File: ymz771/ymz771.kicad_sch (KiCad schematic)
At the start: 94 parts, among them IC1 CH221K, J1 Conn_01x04_Pin, J2 Conn_02x12_Counter_Clockwise, J3 Conn_01x08_Pin, J4 Conn_02x08_Counter_Clockwise, J5 Conn_01x04_Pin, J6 Conn_01x05_Pin, J7 USB_C_Receptacle_PowerOnly_6P, J8 Conn_01x10_Pin, SW1 SW_DIP_x04, Y1 Crystal

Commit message: commit2605161301
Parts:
- removed C10, C7, C8, C9: C_Polarized_Small, Capacitor_THT:CP_Radial_D6.3mm_P2.50mm, symbol Device:C_Polarized_Small
- removed C15, C16: C_Polarized_Small, Capacitor_THT:CP_Radial_D8.0mm_P3.50mm, symbol Device:C_Polarized_Small
- removed D1, D2, D3, D4, D5: LED_Small, LED_SMD:LED_0603_1608Metric_Pad1.05x0.95mm_HandSolder, symbol Device:LED_Small
- removed IC1: CH221K, YMZ771:SOT95P280X120-6N, symbol Yamaha:CH221K
- removed J1: Conn_01x04_Pin, Connector_PinHeader_2.54mm:PinHeader_1x04_P2.54mm_Vertical, symbol Connector:Conn_01x04_Pin
- removed J3: Conn_01x08_Pin, Connector_PinHeader_2.54mm:PinHeader_1x08_P2.54mm_Vertical, symbol Connector:Conn_01x08_Pin
- removed J5: Conn_01x04_Pin, Connector_PinSocket_2.54mm:PinSocket_1x04_P2.54mm_Vertical, symbol Connector:Conn_01x04_Pin
- removed J6: Conn_01x05_Pin, Connector_PinHeader_2.54mm:PinHeader_1x05_P2.54mm_Vertical, symbol Connector:Conn_01x05_Pin
- removed J7: USB_C_Receptacle_PowerOnly_6P, Connector_USB:USB_C_Receptacle_GCT_USB4125-xx-x_6P_TopMnt_Horizontal, symbol Connector:USB_C_Receptacle_PowerOnly_6P
- removed J8: Conn_01x10_Pin, Connector_PinHeader_2.54mm:PinHeader_1x10_P2.54mm_Vertical, symbol Connector:Conn_01x10_Pin
- removed R1, R12, R17, R2, R21, R22, R23, R24, R25, R26, R27, R28, R29, R3, R30, R31, R32, R37, R4, R9: 10k, Resistor_SMD:R_0603_1608Metric_Pad0.98x0.95mm_HandSolder, symbol Device:R_Small
- removed R33: 1k, Resistor_SMD:R_0603_1608Metric_Pad0.98x0.95mm_HandSolder, symbol Device:R_Small
- removed R34, R35: 5.1k, Resistor_SMD:R_0603_1608Metric_Pad0.98x0.95mm_HandSolder, symbol Device:R_Small
- removed R36, R38, R39, R40, R41, R44, R45, R46, R47, R48, R49, R50: 100k, Resistor_SMD:R_0603_1608Metric_Pad0.98x0.95mm_HandSolder, symbol Device:R_Small
- removed SW1: SW_DIP_x04, Button_Switch_SMD:SW_DIP_SPSTx04_Slide_KingTek_DSHP04TS_W7.62mm_P1.27mm, symbol Switch:SW_DIP_x04
- removed U1: ~, YMZ771:YMZ771-F, symbol Yamaha:YMZ771
- removed Y1: Crystal, Crystal:Crystal_SMD_HC49-SD, symbol Device:Crystal
- added C10, C11, C12, C2, C3: 0.1uF, Capacitor_SMD:C_0603_1608Metric, symbol Device:C_Small
- added C14, C15: 2.2nF, Capacitor_SMD:C_0603_1608Metric, symbol Device:C_Small
- added C16, C20: 2.2uF, Capacitor_SMD:C_0603_1608Metric, symbol Device:C_Small
- added C17: 4u7, Capacitor_SMD:C_0603_1608Metric, symbol Device:C
- added C18, C21, C5, C6: 0.1u, Capacitor_SMD:C_0603_1608Metric, symbol Device:C_Small
- added C19, C22, C8, C9: 47u, Capacitor_SMD:C_0603_1608Metric, symbol Device:C_Small
- added C31, C32: C_Small, Capacitor_SMD:C_0603_1608Metric, symbol Device:C_Small
- added C33, C34: 10uF, Capacitor_SMD:C_1812_4532Metric, symbol Device:C_Small
- added C7: 0u1, Capacitor_SMD:C_0603_1608Metric, symbol Device:C
- added D1: LED, LED_SMD:LED_0603_1608Metric, symbol Device:LED
- added D12, D13, D14, D15, D16, D17, D18, D19: LED_Small, LED_SMD:LED_0603_1608Metric_Pad1.05x0.95mm_HandSolder, symbol Device:LED_Small
- added J1: YMZ771-F, QFP80P1880X2480X295-80N, symbol Yamaha:YMZ771-F
- added J2: Micro_SD_Card_Det2, Connector_Card:microSD_HC_Hirose_DM3AT-SF-PEJM5, symbol Connector:Micro_SD_Card_Det2
- added J4: MJ-8435, YMZ771:MJ-8435, symbol Yamaha:MJ-8435
- added J7: USB_C_Receptacle_USB2.0_16P, Connector_USB:USB_C_Receptacle_GCT_USB4105-xx-A_16P_TopMnt_Horizontal, symbol Connector:USB_C_Receptacle_USB2.0_16P
- added J8: Conn_01x02_Pin, Connector_PinHeader_2.54mm:PinHeader_1x02_P2.54mm_Vertical, symbol Connector:Conn_01x02_Pin
- added J9: Conn_02x06_Counter_Clockwise, Connector_PinHeader_1.27mm:PinHeader_2x06_P1.27mm_Vertical_SMD, symbol Connector_Generic:Conn_02x06_Counter_Clockwise
- added Q1, Q2, Q3, Q4: NMOS, Package_TO_SOT_SMD:SOT-23, symbol Transistor_FET_Other:Q_NMOS_Depletion_GSD
- added R1, R3, R4: 5k1, Resistor_SMD:R_0603_1608Metric, symbol Device:R
- added R12, R9: 470, Resistor_SMD:R_0603_1608Metric, symbol Device:R
- added R17: 10k, Resistor_SMD:R_0603_1608Metric, symbol Device:R
- added R55, R56: 10k, Resistor_SMD:R_0603_1608Metric, symbol Device:R_Small
- added RN1, RN10, RN11, RN12, RN13, RN14, RN2, RN3, RN4, RN5, RN6, RN7, RN8, RN9: R_Pack04, Yamaha:MNR04M0ABJ, symbol Device:R_Pack04
- added SW1: SW_Push, footprints:SKRPABE010, symbol Switch:SW_Push
- added SW2: RotaryEncoder, Rotary_Encoder:RotaryEncoder_Bourns_Horizontal_PEC09-2xxxF-Nxxxx, symbol Device:RotaryEncoder
- added SW3: SW_MEC_5E, Yamaha:SW_SKRPABE010, symbol Switch:SW_MEC_5E
- added U1: TS5A23159DGS, Package_SO:VSSOP-10_3x3mm_P0.5mm, symbol Analog_Switch:TS5A23159DGS
- added U10: ESP32-S3-WROOM-1, RF_Module:ESP32-S3-WROOM-1, symbol RF_Module:ESP32-S3-WROOM-1
- added U11, U12: 74AHC541, Package_SO:SSOP-20_5.3x7.2mm_P0.65mm, symbol 74xx:74AHC541
- added U13, U14: (no value), Package_DIP:DIP-8_W7.62mm, symbol Yamaha:PAM8012
- added U2, U5: TXS0104EPW, Package_SO:TSSOP-14_4.4x5mm_P0.65mm, symbol Logic_LevelTranslator:TXS0104EPW
- added U3: (no value), Package_TO_SOT_SMD:TSOT-23-5_HandSoldering, symbol Yamaha:rt9080
- added U4: CH340K, Package_SO:SSOP-10-1EP_3.9x4.9mm_P1mm_EP2.1x3.3mm, symbol Interface_USB:CH340K
- added U6: (no value), YMZ771:OSL2051A-LR, symbol Yamaha:OSL2051A
- added U7: 74HC595, Package_SO:TSSOP-16_4.4x5mm_P0.65mm, symbol 74xx:74HC595
- added U8: PCM5102A, Package_SO:TSSOP-20_4.4x6.5mm_P0.65mm, symbol Audio:PCM5102A
- added Y1: 16.384MHz, Crystal:Crystal_SMD_3225-4Pin_3.2x2.5mm, symbol Device:Crystal_GND24
- C13: value C_Small -> 0.1uF
- J10: renamed from J4; footprint Connector_PinHeader_2.54mm:PinHeader_2x08_P2.54mm_Vertical -> Connector_PinHeader_1.27mm:PinHeader_2x08_P1.27mm_Vertical_SMD
- J11: renamed from J2; footprint Connector_PinHeader_2.54mm:PinHeader_2x12_P2.54mm_Vertical -> Connector_PinHeader_1.27mm:PinHeader_2x12_P1.27mm_Vertical_SMD
- R10, R13, R14, R15, R16, R6, R7, R8: value 10k -> R_Small; footprint Resistor_SMD:R_0603_1608Metric_Pad0.98x0.95mm_HandSolder -> Resistor_SMD:R_0603_1608Metric
- R11, R18, R19, R20, R5: footprint Resistor_SMD:R_0603_1608Metric_Pad0.98x0.95mm_HandSolder -> Resistor_SMD:R_0603_1608Metric
- R51: value 100k -> 1M; footprint Resistor_SMD:R_0603_1608Metric_Pad0.98x0.95mm_HandSolder -> Resistor_SMD:R_0603_1608Metric
- renumbered C6 to C23, C1 to C24, C2 to C25, C14 to C26, C5 to C27, C11 to C28, C12 to C29, C3 to C30, C4 to C35, D7 to D2, D6 to D3, D12 to D4, D13 to D5, D14 to D6, D15 to D7, R43 to R37, R42 to R57
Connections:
- net AVDD is gone; now on net +5V: C25.1
- net VDD1 is gone; now on net +5V: C24.1, R57.2
- net VDD2 is gone; now on net +5V: C27.1, C35.1
- net VDD4 is gone; now on net +5V: C23.1, C28.1
- net /CS is gone; now on an unnamed net: R51.2
- net +5V: now also D2.2 (A), R11.2, R19.2, C10.1, C17.1, C3.2, C33.1, C34.1, C5.2, J1.16 (VDD1), J1.25 (AVDD), J1.28 (~{TEST0}), J1.29 (~{TEST1}), J1.30 (VDD5), J1.37 (~{TEST2}), J1.38 (VDD2), J1.55 (VDD3), J1.72 (VDD4), J7.A4 (VBUS), J7.A9 (VBUS), J7.B4 (VBUS), J7.B9 (VBUS), J8.1 (Pin_1), R1.1, R55.2, R56.2, RN12.5 (R4.2), RN12.6 (R3.2), RN12.7 (R2.2), RN12.8 (R1.2), RN7.5 (R4.2), RN7.6 (R3.2), RN7.7 (R2.2), RN7.8 (R1.2), U1.8 (VCC), U11.20 (VCC), U12.20 (VCC), U13.1 (Vin), U14.1 (Vin), U2.14 (V_{CCB}), U3.1 (Vin), U3.3 (EN), U4.7 (VCC), U5.14 (V_{CCB}), U7.16 (VCC)
- net AD: now also J1.12 (AD), RN8.1 (R1.1), U12.2 (A0)
- net AOL: now also J1.23 (AOL), U1.9
- net AOR: now also J1.24 (AOR), U1.7
- net BCO: now also J1.31 (BCO), U5.11 (B3)
- net CLKO: now also J1.34 (CLKO), U5.10 (B4)
- net ENA: now also J1.13 (ENA), RN8.2 (R2.1), U12.3 (A1)
- net GND: now also R18.1, C10.2, C11.1, C12.2, C14.1, C15.1, C17.2, C18.1, C19.1, C2.1, C20.1, C21.2, C22.2, C3.1, C31.2, C32.2, C33.2, C34.2, C5.1, C6.1, C7.1, C8.1, C9.1, J1.17 (VSS1), J1.26 (AVSS), J1.39 (VSS2), J1.56 (VSS3), J1.73 (VSS4), J2.11 (SHIELD), J2.6 (VSS), J4.2 (2_1), J4.3 (2_2), J7.A1 (GND), J7.A12 (GND), J7.B1 (GND), J7.B12 (GND), J7.S1 (SHIELD), J8.2 (Pin_2), Q1.2 (S), Q2.2 (S), Q3.2 (S), R17.2, R3.1, R4.2, RN1.5 (R4.2), RN1.6 (R3.2), RN1.7 (R2.2), RN1.8 (R1.2), RN10.5 (R4.2), RN10.6 (R3.2), RN10.7 (R2.2), RN10.8 (R1.2), RN11.5 (R4.2), RN11.6 (R3.2), RN11.7 (R2.2), RN11.8 (R1.2), RN13.5 (R4.2), RN13.6 (R3.2), RN13.7 (R2.2), RN13.8 (R1.2), RN14.5 (R4.2), RN14.6 (R3.2), RN14.7 (R2.2), RN14.8 (R1.2), RN2.5 (R4.2), RN2.6 (R3.2), RN2.7 (R2.2), RN2.8 (R1.2), RN3.5 (R4.2), RN3.6 (R3.2), RN3.7 (R2.2), RN3.8 (R1.2), RN4.5 (R4.2), RN4.6 (R3.2), RN4.7 (R2.2), RN4.8 (R1.2), RN5.5 (R4.2), RN5.6 (R3.2), RN5.7 (R2.2), RN5.8 (R1.2), RN6.5 (R4.2), RN6.6 (R3.2), RN6.7 (R2.2), RN6.8 (R1.2), RN8.5 (R4.2), RN8.6 (R3.2), RN8.7 (R2.2), RN8.8 (R1.2), RN9.5 (R4.2), RN9.6 (R3.2), RN9.7 (R2.2), RN9.8 (R1.2), SW1.1, SW2.C, SW3.3 (K), SW3.4 (A), U1.3 (GND), U10.1 (GND), U10.40 (GND), U10.41 (GND), U11.1 (G1), U11.10 (GND), U11.19 (G2), U12.1 (G1), U12.10 (GND), U12.19 (G2), U13.2 (GND), U13.4 (IN-), U13.5 (SPK-), U13.6 (SPK-), U14.2 (GND), U14.4 (IN-), U14.5 (SPK-), U14.6 (SPK-), U2.7 (GND), U3.2 (GND), U4.11 (GND), U4.3 (GND), U5.7 (GND), U7.8 (GND), U8.10 (DEMP), U8.11 (FLT), U8.16 (FMT), U8.19 (DGND), U8.3 (CPGND), U8.9 (AGND), Y1.2, Y1.4; no longer D10.1 (K), D11.1 (K), D2.1 (K), D4.1 (K), D5.1 (K), D6.1 (K), D7.1 (K), D8.1 (K), D9.1 (K), R10.2, R11.2, R13.2, R14.2, R15.2, R16.2, R18.2, R19.2, R20.2, R5.2, R6.2, R7.2, R8.2
- net LRO: now also J1.32 (LRO), U5.13 (B1)
- net MA00: now also J1.65 (MA00), RN1.1 (R1.1)
- net MA01: now also J1.64 (MA01), RN1.2 (R2.1)
- net MA02: now also J1.63 (MA02), RN1.3 (R3.1)
- net MA03: now also J1.62 (MA03), RN1.4 (R4.1)
- net MA04: now also J1.61 (MA04), RN2.1 (R1.1); no longer R5.1
- net MA05: now also J1.60 (MA05), RN2.2 (R2.1); no longer R6.1
- net MA06: now also J1.59 (MA06), RN2.3 (R3.1); no longer R7.1
- net MA07: now also J1.58 (MA07), RN2.4 (R4.1); no longer R8.1
- net MA08: now also J1.57 (MA08), RN3.1 (R1.1)
- net MA09: now also J1.54 (MA09), RN3.2 (R2.1); no longer R10.1
- net MA10: now also J1.53 (MA10), RN3.3 (R3.1); no longer R11.1
- net MA11: now also J1.52 (MA11), RN3.4 (R4.1)
- net MA12: now also J1.51 (MA12), RN4.1 (R1.1); no longer R13.1
- net MA13: now also J1.50 (MA13), RN4.2 (R2.1); no longer R14.1
- net MA14: now also J1.49 (MA14), RN4.3 (R3.1); no longer R15.1
- net MA15: now also J1.48 (MA15), RN4.4 (R4.1); no longer R16.1
- net MA16: now also J1.47 (MA16), RN5.1 (R1.1)
- net MA17: now also J1.46 (MA17), RN5.2 (R2.1); no longer R18.1
- net MA18: now also J1.45 (MA18), RN5.3 (R3.1); no longer R19.1
- net MA19: now also J1.44 (MA19), RN5.4 (R4.1); no longer R20.1
- net MA20: now also J1.43 (MA20), RN6.1 (R1.1)
- net MA21: now also J1.42 (MA21), RN6.2 (R2.1)
- net MA22: now also J1.41 (MA22), RN6.3 (R3.1)
- net MA23: now also J1.40 (MA23), RN6.4 (R4.1)
- net MBMD: now also J1.20 (MBMD), RN7.3 (R3.1), U12.8 (A6)
- net MD00: now also J1.3 (MD00)
- net MD01: now also J1.2 (MD01)
- net MD02: now also J1.1 (MD02)
- net MD03: now also J1.80 (MD03)
- net MD04: now also J1.79 (MD04)
- net MD05: now also J1.78 (MD05)
- net MD06: now also J1.77 (MD06)
- net MD07: now also J1.76 (MD07)
- net MD08: now also J1.75 (MD08)
- net MD09: now also J1.74 (MD09)
- net MD10: now also J1.71 (MD10)
- net MD11: now also J1.70 (MD11)
- net MD12: now also J1.69 (MD12)
- net MD13: now also J1.68 (MD13)
- net MD14: now also J1.67 (MD14)
- net MD15: now also J1.66 (MD15)
- net SDO: now also J1.33 (SDO), U5.12 (B2)
- net +3V3: now reaches C13.1
- net +3V3: now also R20.2, C11.2, C12.1, C2.2, C21.1, C22.1, C6.2, C8.2, C9.2, J2.4 (VDD), Q4.1 (G), U10.2 (3V3), U2.1 (V_{CCA}), U2.8 (OE), U3.5 (Vout), U5.1 (V_{CCA}), U5.8 (OE), U8.1 (CPVDD), U8.20 (DVDD), U8.8 (AVDD)
- net at D9.2 (A): now also RN12.2 (R2.1)
- net at D6.2 (A): now also U12.16 (Y2)
- net at D10.2 (A): now also RN12.3 (R3.1)
- net at C30.1: now also R51.1, J1.36 (XI), Y1.1
- net at D4.2 (A): now also U12.18 (Y0)
- net at C29.1: now also J1.35 (XO), Y1.3
- net at R37.1: now also D2.1 (K); no longer D2.2 (A)
- net at D8.2 (A): now also RN12.1 (R1.1)
- net at D11.2 (A): now also RN12.4 (R4.1)
- net at D5.2 (A): now also U12.17 (Y1)
- net at D7.2 (A): now also U12.15 (Y3); no longer R51.1
- net Vref: no longer names the net of C26.1
- net Vref: now also J1.27 (VREF)
- net /PLAY renamed /PLAY#
- net /PLAY#: now also R19.1, J1.22 (~{PLAY}), Q4.3 (D)
- new net: D19.1 (K), RN10.4 (R4.1)
- new net: D19.2 (A), U11.11 (Y7)
- new net: R9.2, U8.6 (OUTL)
- new net: R7.1, U7.1 (QB)
- new net: R7.2, U6.9 (B)
- new net: C20.2, U8.5 (VNEG)
- new net: R14.1, U7.5 (QF)
- new net: R14.2, U6.7 (F)
- new net: R6.1, U7.15 (QA)
- new net: R8.1, U7.2 (QC)
- new net: R10.1, U7.3 (QD)
- new net: R13.1, U7.4 (QE)
- new net: R15.1, U7.6 (QG)
- new net: R16.1, U7.7 (QH)
- new net: Q1.1 (G), R5.1
- new net: R10.2, U6.1 (D)
- new net: D6.1 (K), RN11.3 (R3.1)
- new net: D16.1 (K), RN10.1 (R1.1)
- new net: D16.2 (A), U11.14 (Y4)
- new net: J7.A5 (CC1), R3.2
- new net: J4.4 (3), U14.7 (SPK+), U14.8 (SPK+)
- new net: D12.1 (K), RN9.1 (R1.1)
- new net: D12.2 (A), U11.18 (Y0)
- new net: D1.1 (K), R17.1
- new net: Q2.3 (D), U6.10 (DIG1)
- new net: R16.2, U6.2 (DP)
- new net: R15.2, U6.3 (G)
- new net: R13.2, U6.4 (E)
- new net: Q3.3 (D), U6.5 (DIG2)
- new net: R6.2, U6.6 (A)
- new net: R8.2, U6.8 (C)
- new net: Q1.3 (D), Q2.1 (G), R11.1
- new net: D15.1 (K), RN9.4 (R4.1)
- new net: D15.2 (A), U11.15 (Y3)
- new net: D4.1 (K), RN11.1 (R1.1)
- new net: D17.1 (K), RN10.2 (R2.1)
- new net: D18.1 (K), RN10.3 (R3.1)
- new net: C18.2, C19.2, U8.18 (LDOO)
- new net: Q4.2 (S), R20.1, U8.17 (XSMT)
- new net: C7.2, U4.10 (V3)
- new net: D8.1 (K), U12.14 (Y4)
- new net: D9.1 (K), U12.13 (Y5)
- new net: J4.1, U13.7 (SPK+), U13.8 (SPK+)
- new net: J7.B5 (CC2), R4.1
- new net: D13.1 (K), RN9.2 (R2.1)
- new net: D14.1 (K), RN9.3 (R3.1)
- new net: D18.2 (A), U11.12 (Y6)
- new net: D17.2 (A), U11.13 (Y5)
- new net: D14.2 (A), U11.16 (Y2)
- new net: D13.2 (A), U11.17 (Y1)
- new net: U5.5 (A4), U8.12 (SCK)
- new net: U5.4 (A3), U8.13 (BCK)
- new net: U5.3 (A2), U8.14 (DIN)
- new net: U5.2 (A1), U8.15 (LRCK)
- new net: C16.1, U8.2 (CAPP)
- new net: C16.2, U8.4 (CAPM)
- new net: R12.2, U8.7 (OUTR)
- new net: D5.1 (K), RN11.2 (R2.1)
- new net: D10.1 (K), U12.12 (Y6)
- new net: J2.7 (DAT0), U2.2 (A1)
- new net: J2.5 (CLK), U2.3 (A2)
- new net: J2.3 (CMD), U2.4 (A3)
- new net: J2.2 (DAT3/CD), U2.5 (A4)
- new net: D11.1 (K), U12.11 (Y7)
- new net: D7.1 (K), RN11.4 (R4.1)
- new net 7seg: Q3.1 (G), R18.2, R5.2
- new net D+: J7.A6 (D+), J7.B6 (D+), U4.1 (UD+)
- new net D-: J7.A7 (D-), J7.B7 (D-), U4.2 (UD-)
- new net MISO: U2.13 (B1)
- new net MOSI: U2.11 (B3)
- new net OUTL: C14.2, R9.1, U1.2
- new net OUTR: C15.2, R12.1, U1.4
- new net PA0: J1.21 (~{RESET}), RN7.4 (R4.1), U12.9 (A7)
- new net PA2: J1.19 (~{SEL}), RN7.2 (R2.1), U12.7 (A5)
- new net PA3: J1.18 (S6M), RN7.1 (R1.1), U12.6 (A4)
- new net PA4: J1.15 (~{CS}), RN8.4 (R4.1), U12.5 (A3)
- new net PA5: J1.14 (~{WR}), RN8.3 (R3.1), U12.4 (A2)
- new net PB0: C32.1, R56.1, SW2.A
- new net PB1: C31.1, R55.1, SW2.B
- new net PB2: J9.12 (Pin_12)
- new net PB3: J9.11 (Pin_11)
- new net PB4: J9.10 (Pin_10)
- new net PB5: J9.9 (Pin_9)
- new net PC0: J1.4 (CD0), RN14.1 (R1.1), U11.2 (A0)
- new net PC1: J1.5 (CD1), RN14.2 (R2.1), U11.3 (A1)
- new net PC2: J1.6 (CD2), RN14.3 (R3.1), U11.4 (A2)
- new net PC3: J1.7 (CD3), RN14.4 (R4.1), U11.5 (A3)
- new net PC4: J1.8 (CD4), RN13.1 (R1.1), U11.6 (A4)
- new net PC5: J1.9 (CD5), RN13.2 (R2.1), U11.7 (A5)
- new net PC6: J1.10 (CD6), RN13.3 (R3.1), U11.8 (A6)
- new net PC7: J1.11 (CD7), RN13.4 (R4.1), U11.9 (A7)
- new net PD0: J9.6 (Pin_6)
- new net PD1: J9.5 (Pin_5)
- new net PD2: J9.4 (Pin_4)
- new net PD3: J9.3 (Pin_3)
- new net PD4: J9.2 (Pin_2)
- new net PD5: J9.1 (Pin_1)
- new net PD6: J9.7 (Pin_7)
- new net PD7: J9.8 (Pin_8)
- new net PF1: U7.13 (~{OE})
- new net PF2: U7.12 (RCLK)
- new net PF3: SW1.2
- new net PF4: U7.10 (~{SRCLR})
- new net PF5: U7.11 (SRCLK)
- new net PF6: U7.14 (SER)
- new net SCK: U2.12 (B2)
- new net SP: R1.2, SW3.1, SW3.2, U1.1, U1.5
- new net SPL: U1.10, U13.3 (IN+)
- new net SPR: U1.6, U14.3 (IN+)
- new net SS: U2.10 (B4)
- new net TNOW: D1.2 (A), U4.4 (~{DTR})
- new net UPDI/340K: U4.8 (TXD), U4.9 (RXD)
- no-connect marks 0 -> 8
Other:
- note added: "5v to 3.3v"
- note added: "7Segment"
- note added: "Encoder"
- note added: "I2S DAC"
- note added: "LED BUS"
- note added: "MCU"
- note added: "SD Slot"
- note added: "SP jack"
- note added: "USB-Serial"
- note added: "YMZ771"
- moved on the sheet: C23, C24, C25, C26, C27, C28, C29, C30, C35, D10, D11, D2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

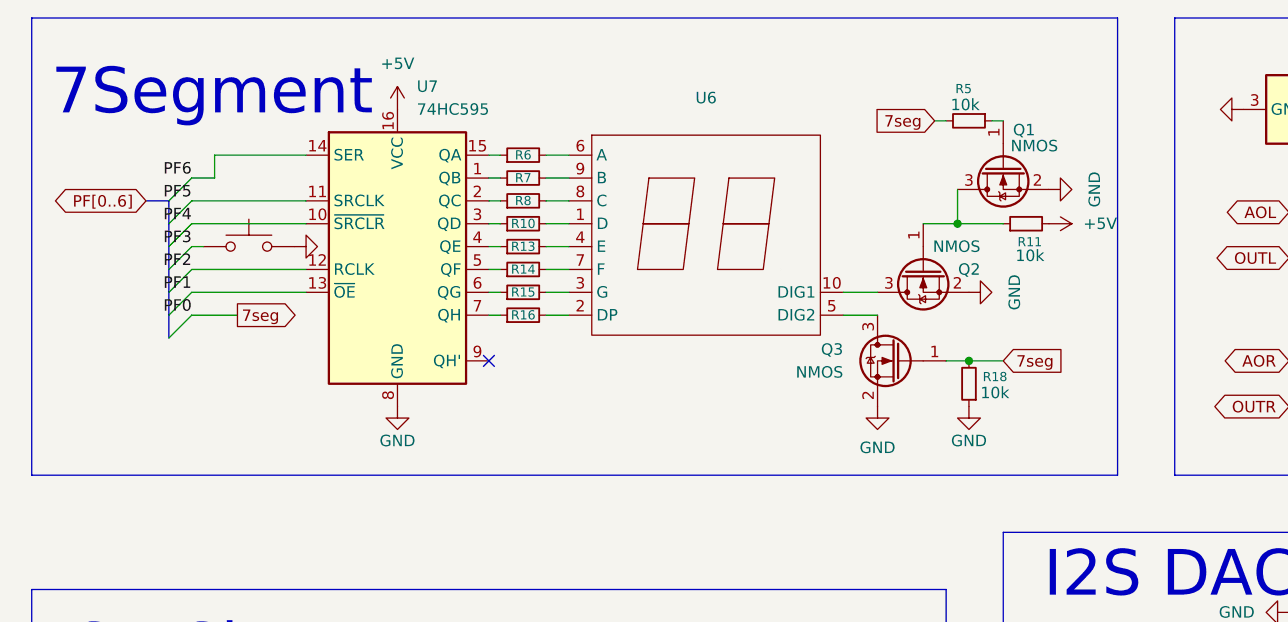
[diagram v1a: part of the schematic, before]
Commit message: 2605181741
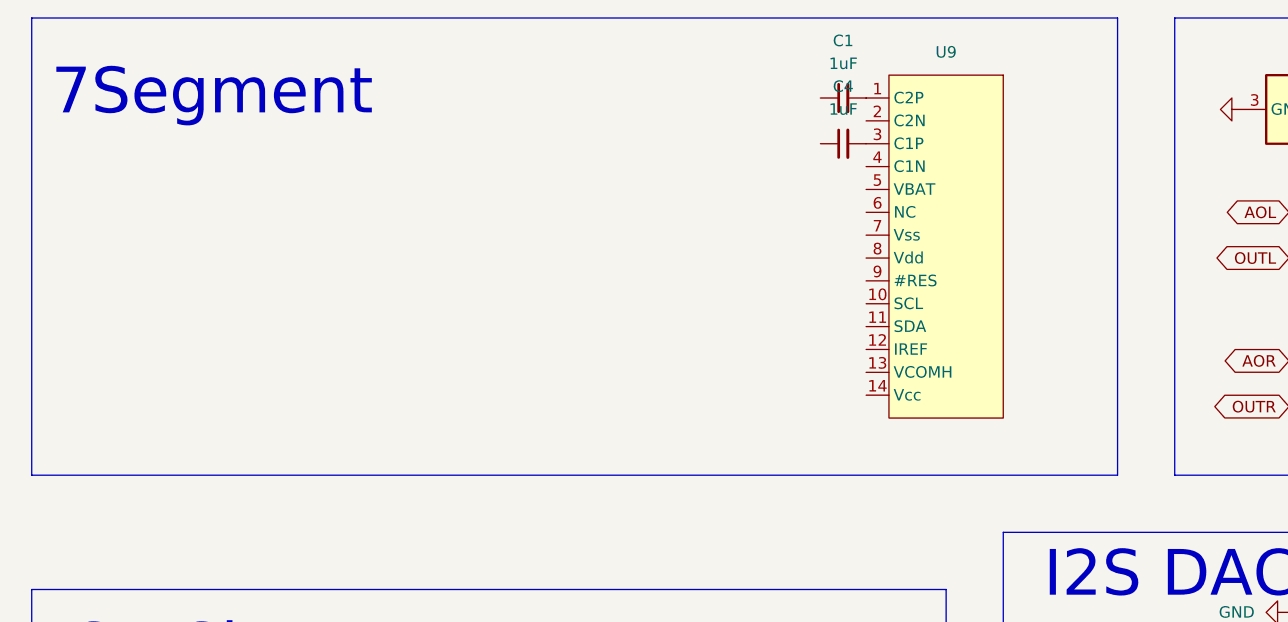
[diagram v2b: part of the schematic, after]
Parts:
- removed Q1, Q2, Q3: NMOS, Package_TO_SOT_SMD:SOT-23, symbol Transistor_FET_Other:Q_NMOS_Depletion_GSD
- removed R10, R13, R14, R15, R16, R6, R7, R8: R_Small, Resistor_SMD:R_0603_1608Metric, symbol Device:R_Small
- removed R11, R18, R5: 10k, Resistor_SMD:R_0603_1608Metric, symbol Device:R_Small
- removed SW1: SW_Push, footprints:SKRPABE010, symbol Switch:SW_Push
- removed U6: (no value), YMZ771:OSL2051A-LR, symbol Yamaha:OSL2051A
- removed U7: 74HC595, Package_SO:TSSOP-16_4.4x5mm_P0.65mm, symbol 74xx:74HC595
- added C1, C4: 1uF, symbol Device:C_Small
- added U9: (no value), symbol Yamaha:X032-6032TSWAG02-H14
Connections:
- new net: C1.2, U9.1 (C2P)
- new net: C4.2, U9.3 (C1P)
- no-connect marks 8 -> 7
